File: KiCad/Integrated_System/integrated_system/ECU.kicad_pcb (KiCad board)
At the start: 2 copper layers, 106.5 x 81 mm, 50 parts, among them J1 Jack-DC, J2 Fan 1, J3 Fan 2, J4 Fan 3, Q1 BSS138, Q2 BSS138, Q3 BSS138, SW1 SW_SPDT, SW2 SW_SPDT, SW3 SW_Push, U1 SGP30, U2 BME680, U4 Mini360 DC to DC Buck Convert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, U5 SCD30

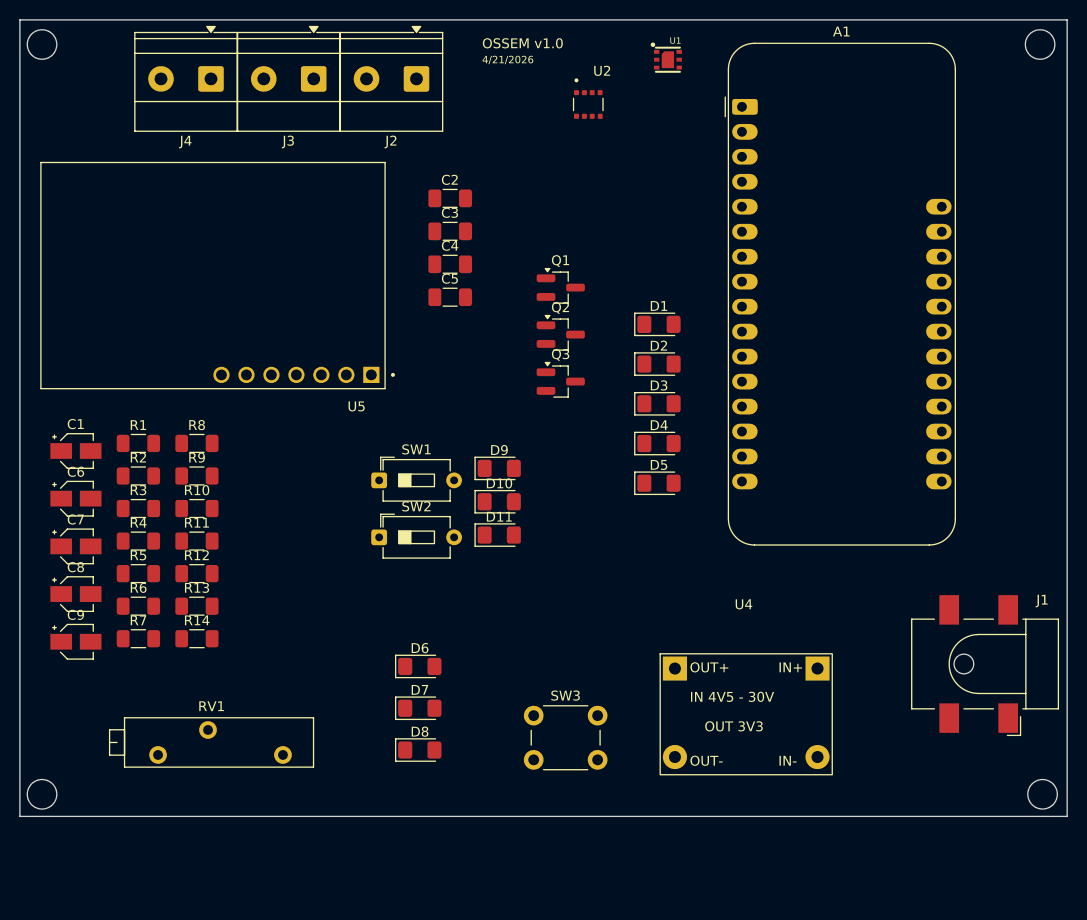
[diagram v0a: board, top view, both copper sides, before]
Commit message: Rough Board layout
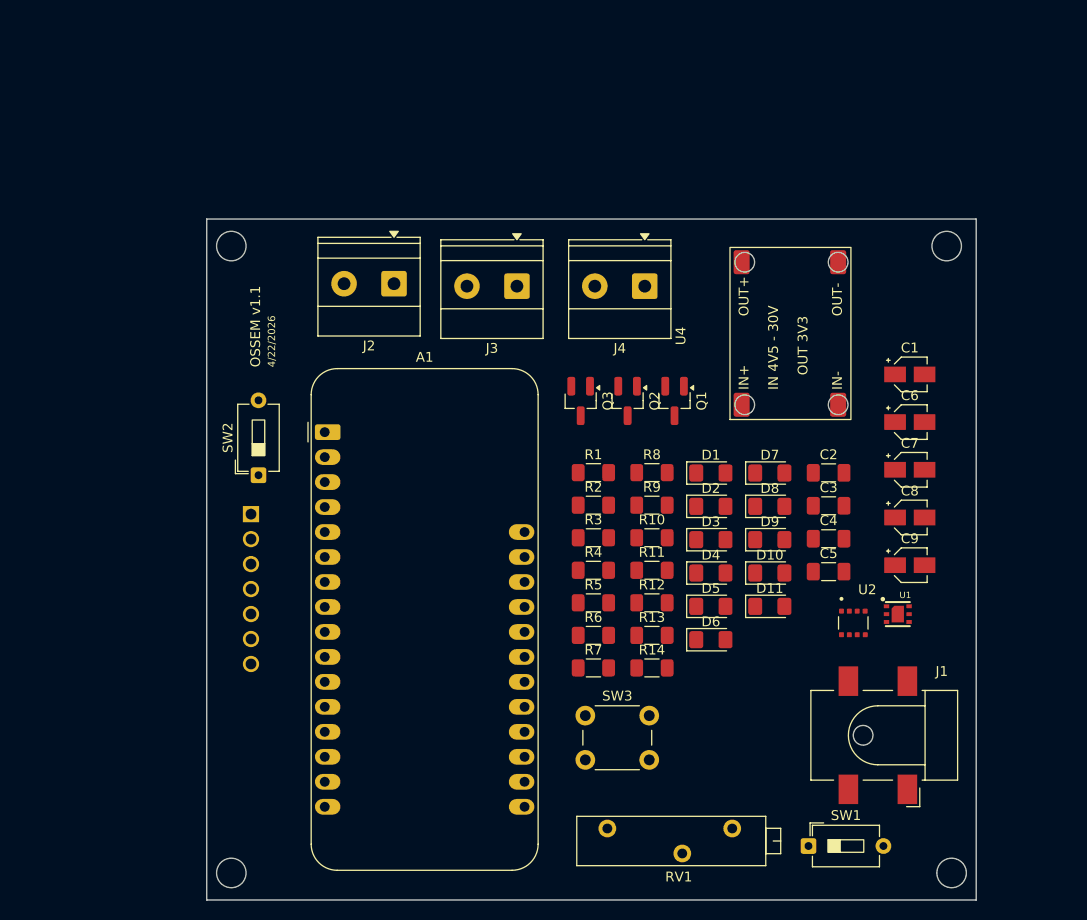
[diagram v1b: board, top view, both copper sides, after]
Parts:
- U5: moved to B.Cu
- moved C1 85.2 mm to (193.0, 78.0)
- moved C6 85.2 mm to (193.0, 82.9)
- moved C7 85.2 mm to (193.0, 87.8)
- moved C8 85.2 mm to (193.0, 92.6)
- moved C9 85.2 mm to (193.0, 97.5)
- moved U1 61.0 mm to (191.8, 102.4)
- moved U2 59.2 mm to (187.2, 103.3)
- moved SW1 57.4 mm to (182.7, 126.0)
- moved A1 53.8 mm to (133.5, 83.9)
- moved J4 48.9 mm to (166.0, 69.1)
- moved C2 47.5 mm to (184.7, 88.1)
- moved C4 47.5 mm to (184.7, 94.8)
- moved C3 47.5 mm to (184.7, 91.4)
- moved C5 47.5 mm to (184.7, 98.1)
- moved R10 46.4 mm to (166.8, 94.7)
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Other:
- board size 106.5 x 81 mm -> 78.2 x 69.2 mm
- board text added: "4/22/2026"
- board text added: "OSSEM v1.1"
- board text removed: "4/21/2026"
- board text removed: "OSSEM v1.0"
